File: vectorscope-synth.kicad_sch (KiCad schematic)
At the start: 22 parts, among them J1 STYLUS, J2 IO CONNECTOR, J3 SCOPE, J4 SIGGEN, J5 PATCH SELECT, J6 WRITE PATCH, J7 PARAM SELECT, J8 MODE, SW1 SW_SPST, SW2 SW_SPST, U1 stm32f103c8t6-module-china

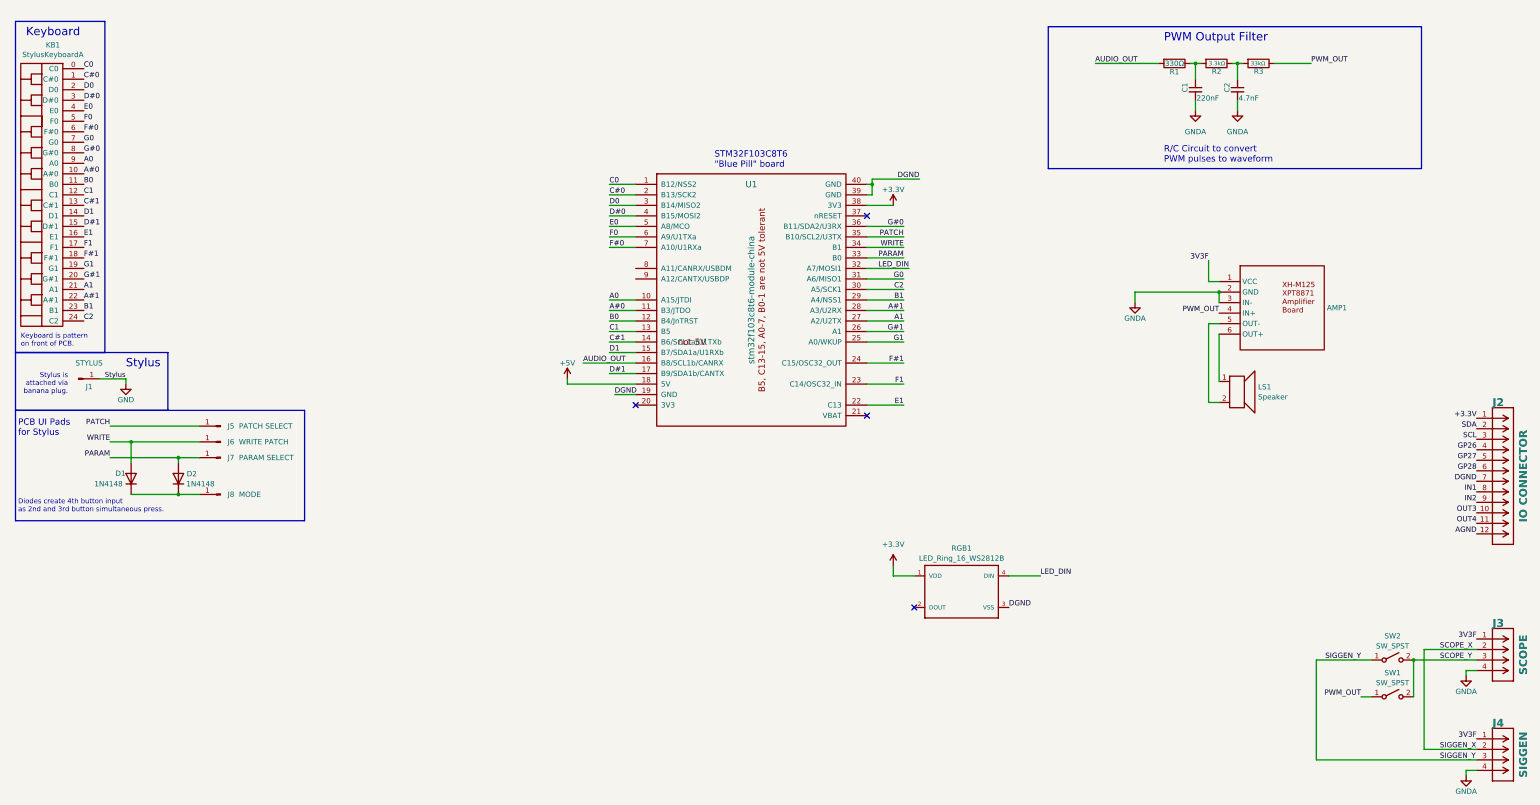
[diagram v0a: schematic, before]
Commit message: Credits, and schematic PDF
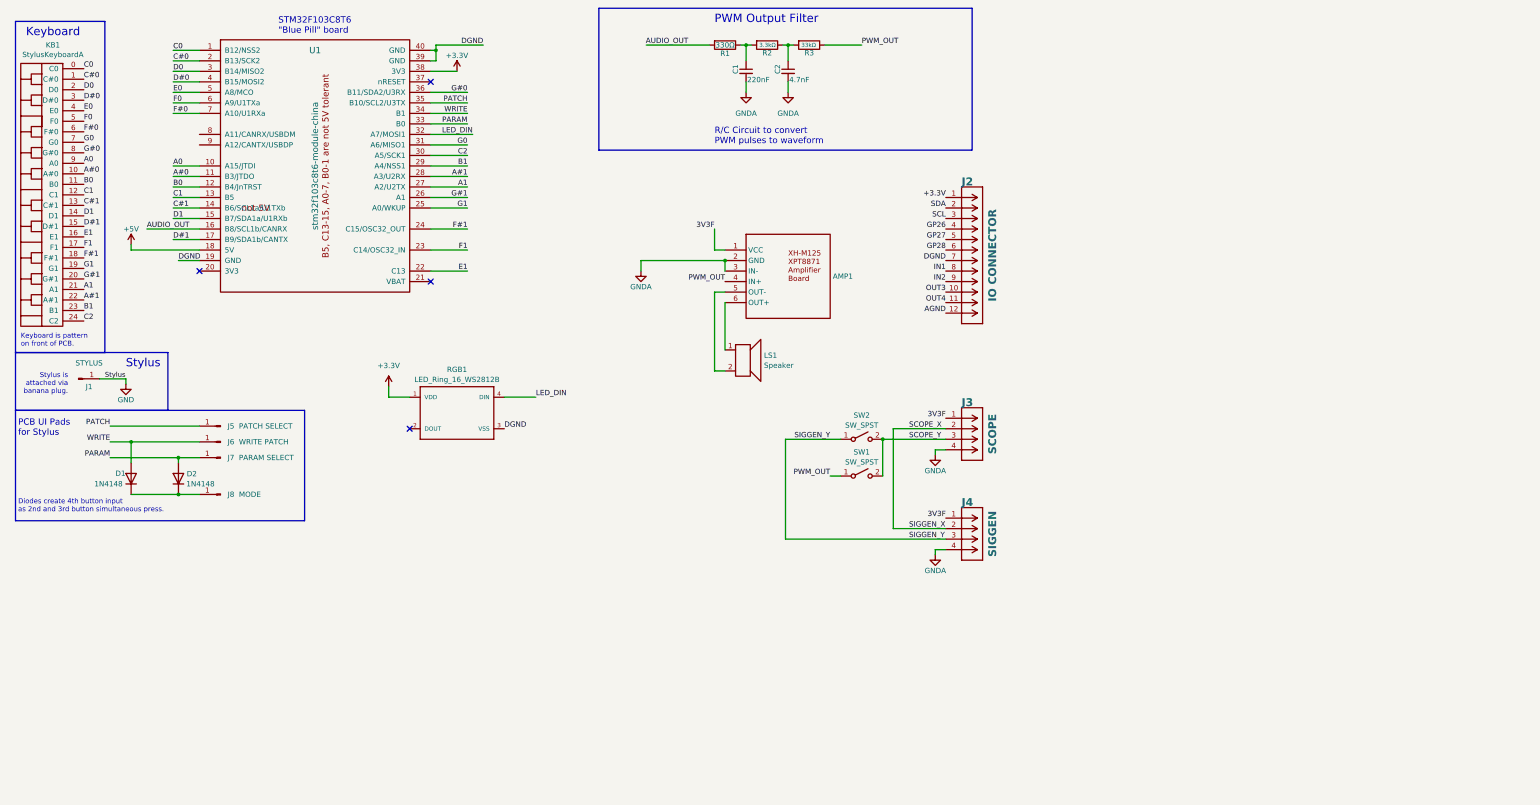
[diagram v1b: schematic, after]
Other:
- moved on the sheet: AMP1, C1, C2, J2, J3, J4, LS1, R1, R2, R3, RGB1, SW1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
